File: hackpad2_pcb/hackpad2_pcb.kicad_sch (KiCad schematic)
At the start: 2 parts, among them U1 MOUDLE-SEEEDUINO-XIAO

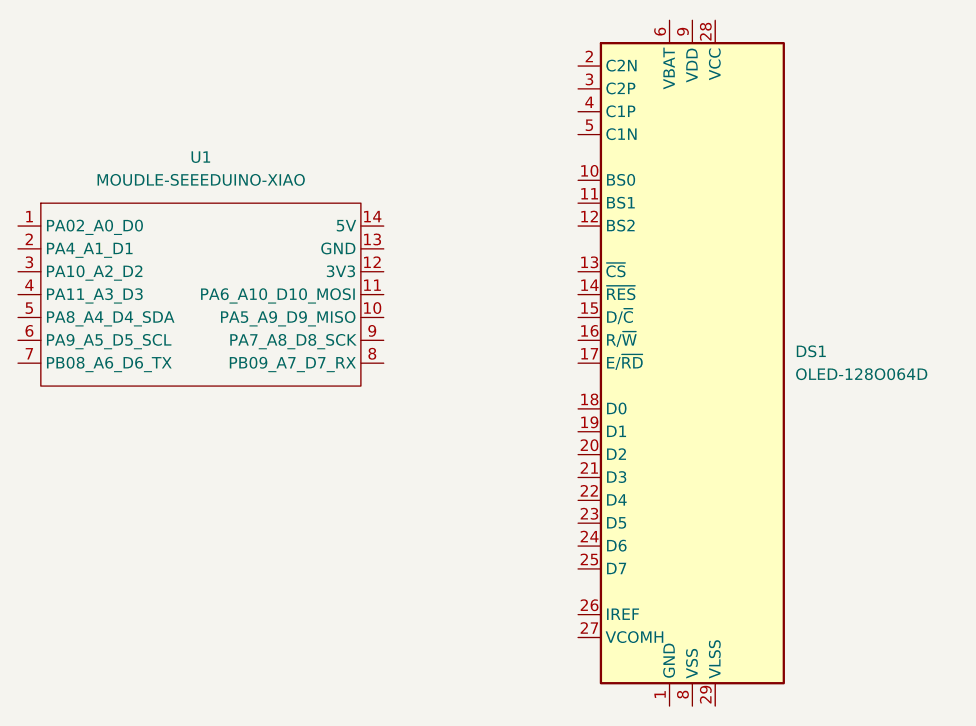
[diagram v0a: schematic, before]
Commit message: oled
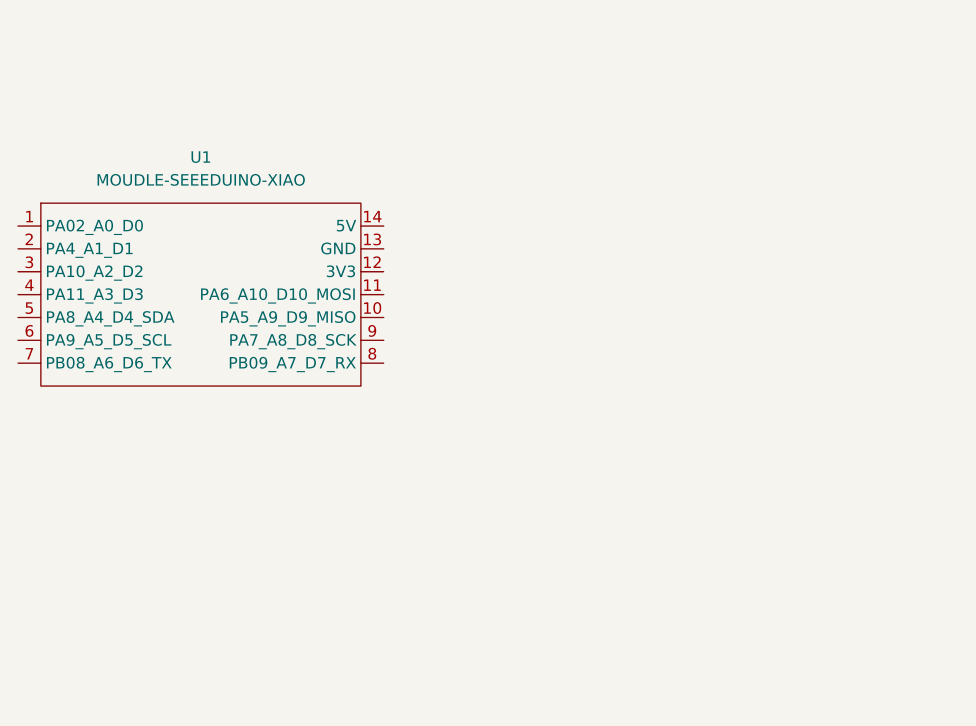
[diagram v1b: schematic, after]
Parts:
- removed DS1: OLED-128O064D, Display:OLED-128O064D, symbol Display_Graphic:OLED-128O064D
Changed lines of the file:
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@@
 	(paper "A4")
-	(symbol
-		(lib_id "Display_Graphic:OLED-128O064D")
-		(at 106.68 80.01 0)
-		(unit 1)
-		(body_style 1)
-		(exclude_from_sim no)
-		(in_bom yes)
-		(on_board yes)
-		(in_pos_files yes)
-		(dnp no)
-		(fields_autoplaced yes)
-		(property "Reference" "DS1"
-			(at 118.11 78.7399 0)
-			(show_name no)
-			(do_not_autoplace no)
-			(effects
-				(font
-					(size 1.27 1.27)
-				)
-				(justify left)
-			)
-		)
-		(property "Value" "OLED-128O064D"
-			(at 118.11 81.2799 0)
-			(show_name no)
-			(do_not_autoplace no)
-			(effects
-				(font
-					(size 1.27 1.27)
-				)
-				(justify left)
-			)
-		)
-		(property "Footprint" "Display:OLED-128O064D"
-			(at 106.68 80.01 0)
-			(hide yes)
-			(show_name no)
-			(do_not_autoplace no)
-			(effects
-				(font
-					(size 1.27 1.27)
-				)
-			)
-		)
-		(property "Datasheet" "https://www.vishay.com/docs/37902/oled128o064dbpp3n00000.pdf"
-			(at 106.68 59.69 0)
-			(hide yes)
-			(show_name no)
-			(do_not_autoplace no)
-			(effects
-				(font
-					(size 1.27 1.27)
-				)
-			)
-		)
-		(property "Description" "OLED display 128x64"
-			(at 106.68 80.01 0)
-			(hide yes)
-			(show_name no)
-			(do_not_autoplace no)
-			(effects
-				(font
-					(size 1.27 1.27)
-				)
-			)
-		)
-		(pin "10"
-		)
-		(pin "30"
-		)
-		(pin "5"
-		)
-		(pin "6"
-		)
-		(pin "13"
-		)
-		(pin "19"
-		)
-		(pin "23"
-		)
-		(pin "28"
-		)
-		(pin "29"
-		)
-		(pin "9"
-		)
-		(pin "16"
-		)
-		(pin "4"
-		)
-		(pin "26"
-		)
-		(pin "27"
-		)
-		(pin "25"
-		)
-		(pin "20"
-		)
-		(pin "21"
-		)
-		(pin "8"
-		)
-		(pin "2"
-		)
-		(pin "3"
-		)
-		(pin "17"
-		)
-		(pin "1"
-		)
-		(pin "14"
-		)
-		(pin "7"
-		)
-		(pin "22"
-		)
-		(pin "12"
-		)
-		(pin "11"
-		)
-		(pin "24"
-		)
-		(pin "15"
-		)
-		(pin "18"
-		)
-		(instances
-			(project "hackpad2_pcb"
-				(path "/bb22a1ff-aa67-456c-b4ba-d8fa4da2229e"
-					(reference "DS1")
-					(unit 1)
-				)
-			)
-		)
-	)
 	(symbol
 		(lib_id "XIAO_RP2040:MOUDLE-SEEEDUINO-XIAO")
